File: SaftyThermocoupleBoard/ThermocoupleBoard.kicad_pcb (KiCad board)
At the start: 4 copper layers, 62.6 x 50.4 mm, 62 parts, among them J2 1935161, J3 1935161, J4 1935161, J5 Conn_01x20_Pin, U1 LT1962-3.3, U2 MAX31856, U3 MAX31856, U4 MAX31856

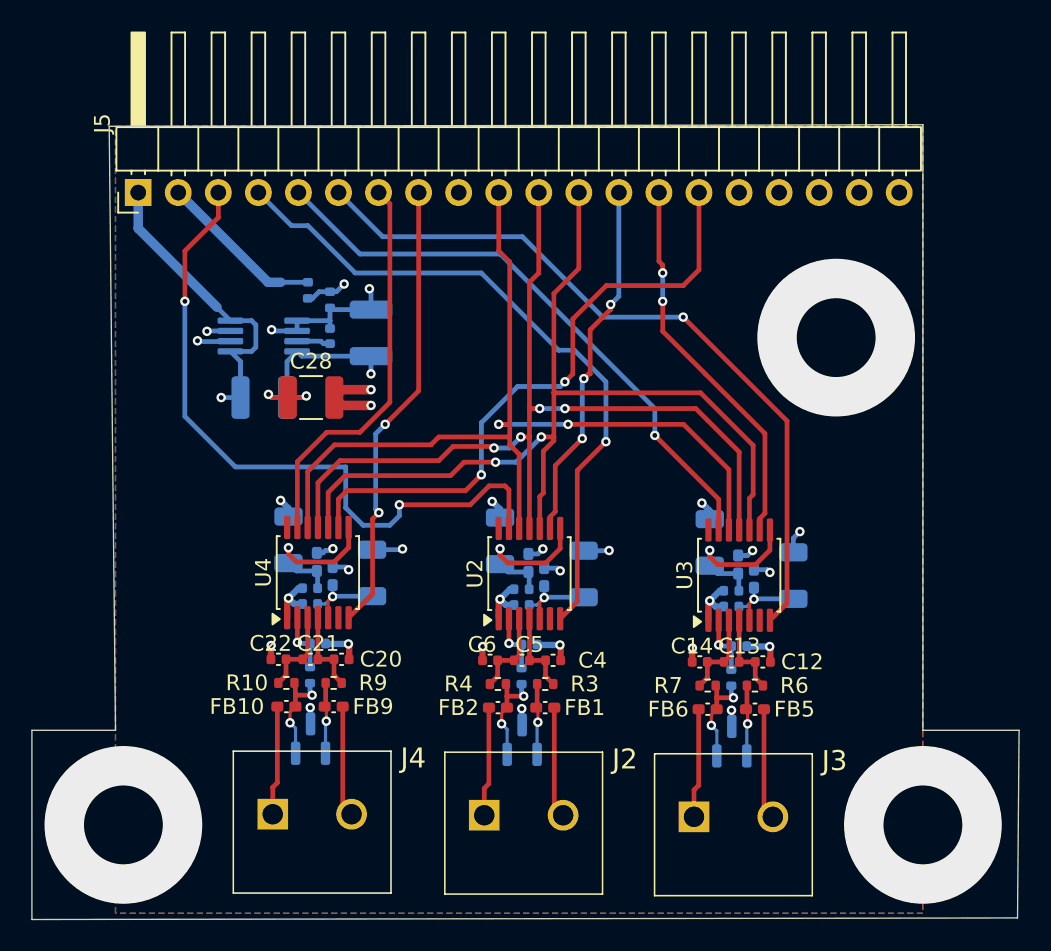
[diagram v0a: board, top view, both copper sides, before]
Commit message: add single thermocouple board
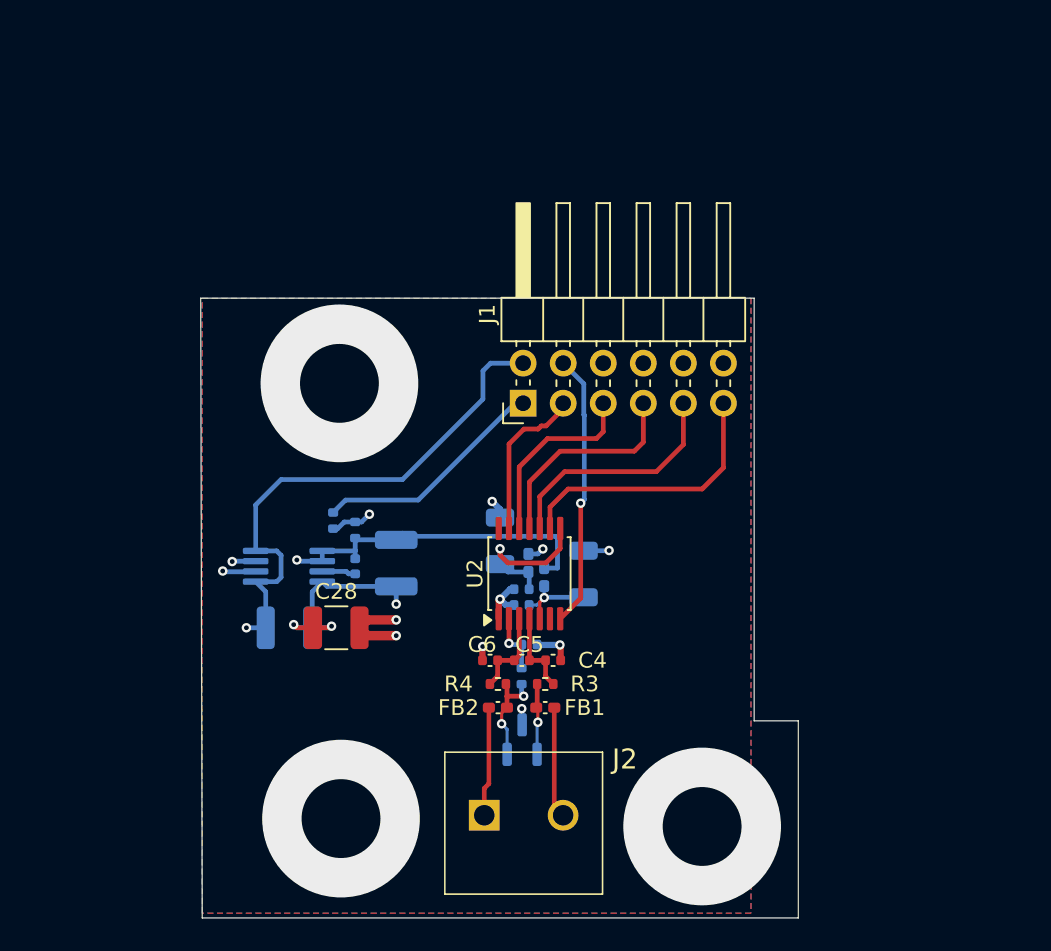
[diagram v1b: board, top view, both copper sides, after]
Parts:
- removed C12, C14, C15, C20, C22, C23: 0.01uf, Capacitor_SMD:C_0402_1005Metric
- removed C13, C17, C19, C21, C25, C27: 0.1uf, Capacitor_SMD:C_0402_1005Metric
- removed C16, C18, C24, C26: 2.2uF, Capacitor_SMD:C_1206_3216Metric
- removed D2, D3: NUP2105L, Package_TO_SOT_SMD:SOT-23
- removed FB10, FB11, FB12, FB5, FB6, FB7, FB8, FB9: 1.8k, Inductor_SMD:L_0402_1005Metric_Pad0.77x0.64mm_HandSolder
- removed J3, J4: 1935161, SamacSys_Parts:1935161
- removed J5: Conn_01x20_Pin, Connector_PinHeader_2.54mm:PinHeader_1x20_P2.54mm_Horizontal
- removed R10, R11, R6, R7, R8, R9: 2.2k, Resistor_SMD:R_0402_1005Metric
- removed U3, U4: MAX31856, Package_SO:TSSOP-14_4.4x5mm_P0.65mm
- added J1: Conn_02x06_Odd_Even, Connector_PinHeader_2.54mm:PinHeader_2x06_P2.54mm_Horizontal, F.Cu at (94.2, 110.3)
- moved C3 14.7 mm to (86.1, 120.4)
- moved R2 14.7 mm to (82.1, 117.7)
- moved C1 14.7 mm to (79.3, 124.5)
- moved C2 14.7 mm to (83.5, 120.6)
- moved C28 14.7 mm to (82.3, 124.5)
- moved R1 14.7 mm to (83.5, 118.3)
- moved U1 14.7 mm to (79.3, 120.6)
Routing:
- net /thermoDrdy_1: track 47.5 -> 0.00 mm, vias 1 -> 0
- net /MOSI: track 59.4 -> 12.0 mm, vias 2 -> 0
- net /MISO: track 58.5 -> 13.7 mm, vias 4 -> 0
- net /CLK: track 59.8 -> 15.1 mm, vias 2 -> 0
- net /CS2: track 39.6 -> 0.00 mm, vias 2 -> 0
- net /thermoFault_1: track 37.7 -> 0.00 mm, vias 1 -> 0
- net /thermoFault_0: track 44.0 -> 10.1 mm, vias 2 -> 0
- net 3.3V_A: track 59.4 -> 29.1 mm, vias 5 -> 1
- net /thermoDrdy_2: track 29.0 -> 0.00 mm, vias 2 -> 0
- net 3.3_D: track 57.5 -> 29.8 mm, vias 6 -> 4
- net /thermoDrdy_0: track 43.2 -> 17.4 mm
- net /thermoFault_2: track 25.2 -> 0.00 mm
- net /CS1: track 24.3 -> 0.00 mm, vias 2 -> 0
- net GND: track 46.4 -> 24.9 mm, vias 21 -> 9
- net 5V: track 19.8 -> 33.9 mm
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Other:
- board size 62.6 x 50.4 mm -> 37.9 x 39.3 mm
